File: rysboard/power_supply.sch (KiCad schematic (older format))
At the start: 31 parts, among them J19 Fan_Connector, Q3 NST847BDP6T5G, Q4 DMP3036SSD-13, Q5 DMP3036SSD-13, U3 ST1S10, U6 L78L33_SO8

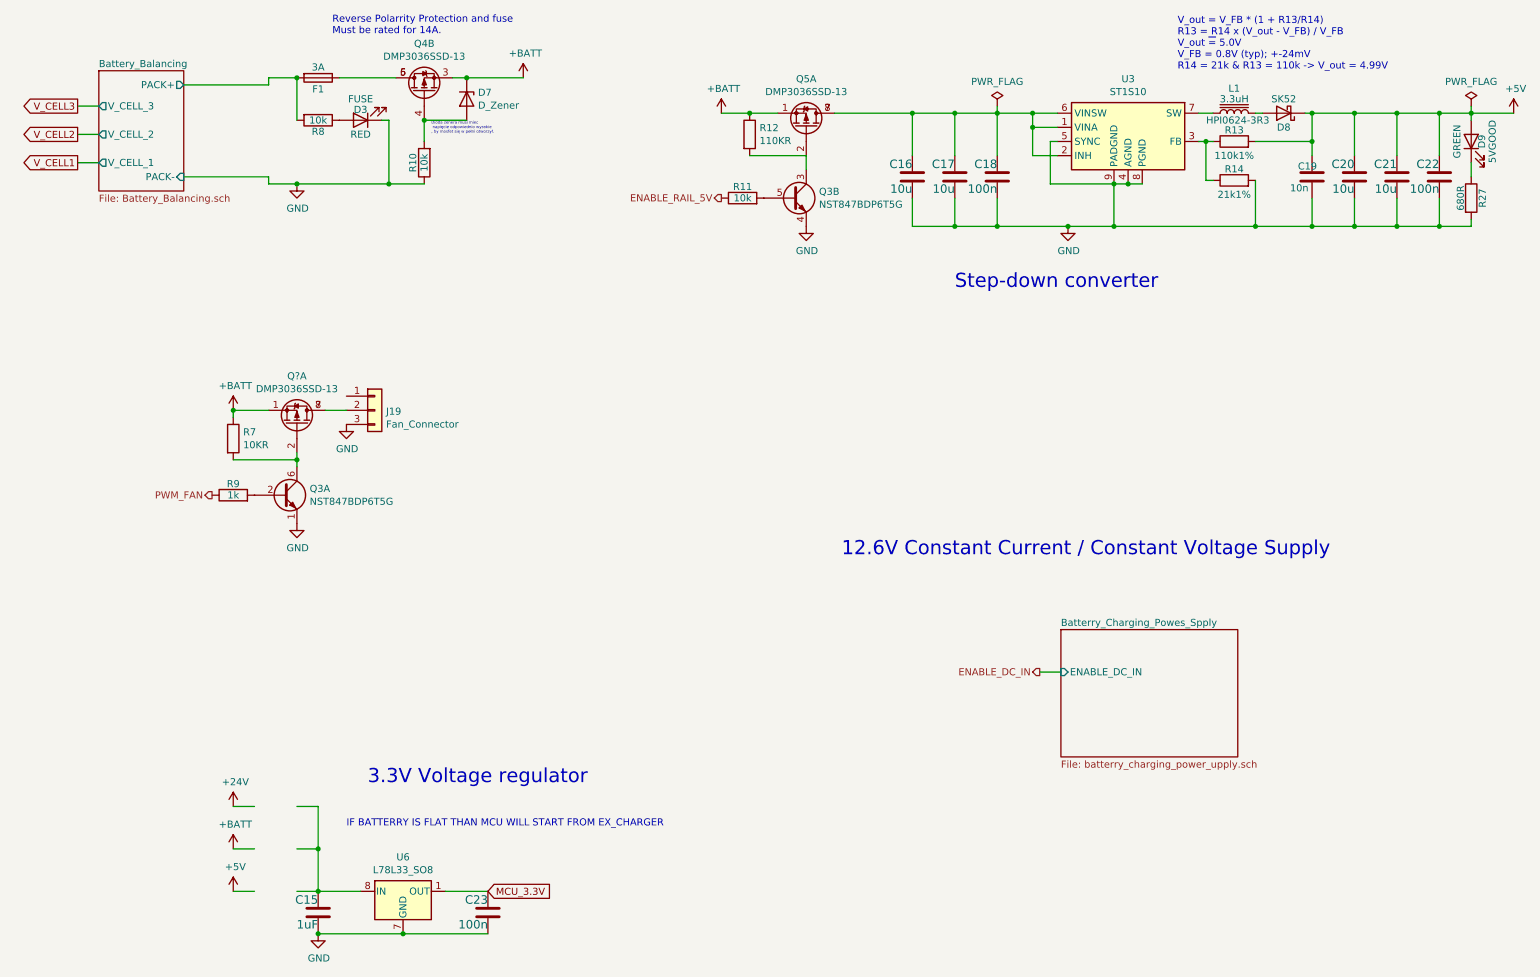
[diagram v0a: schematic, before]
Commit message: more work done
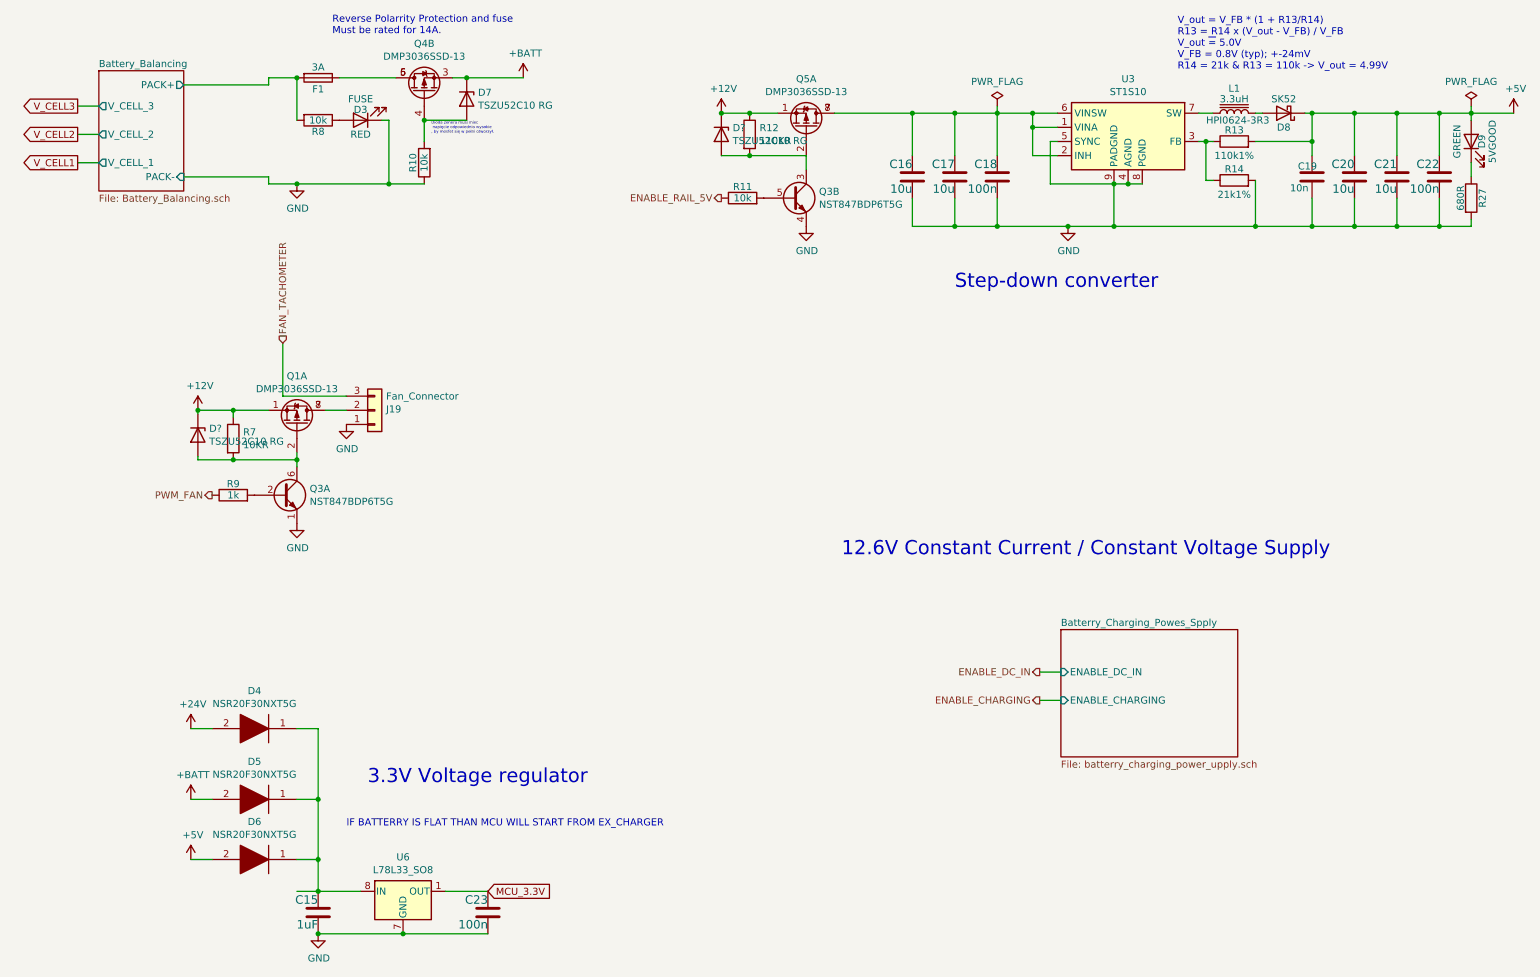
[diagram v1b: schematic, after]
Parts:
- added D4, D5, D6: NSR20F30NXT5G, DSN2_1, symbol SamacSys_Parts:NSR20F30NXT5G
- added D? (x2): TSZU52C10 RG, Diode_SMD:D_0603_1608Metric, symbol Device:D_Zener
- D7: value D_Zener -> TSZU52C10 RG; footprint (none) -> Diode_SMD:D_0603_1608Metric
- gave numbers to parts that had none: 1
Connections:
- net labels added: +12V, ENABLE_CHARGING, FAN_TACHOMETER
- wire segments 101 -> 111
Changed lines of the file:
@@
 P 3600 1250
 F 0 "D7" V 3554 1330 50  0000 L CNN
-F 1 "D_Zener" V 3645 1330 50  0000 L CNN
-F 2 "" H 3600 1250 50  0001 C CNN
+F 1 "TSZU52C10 RG" V 3645 1330 50  0000 L CNN
+F 2 "Diode_SMD:D_0603_1608Metric" H 3600 1250 50  0001 C CNN
 F 3 "~" H 3600 1250 50  0001 C CNN
 	1    3600 1250
@@
 Text Notes 2650 800  0    50   ~ 0
 Reverse Polarrity Protection and fuse\nMust be rated for 14A.\n
-Wire Wire Line
-	2400 6550 2550 6550
-Wire Wire Line
-	2550 6550 2550 6850
 Text Notes 2750 6400 0    50   ~ 0
 IF BATTERRY IS FLAT THAN MCU WILL START FROM EX_CHARGER\n
@@
 F1 "batterry_charging_power_upply.sch" 50
 F2 "ENABLE_DC_IN" I L 7800 5300 50
+F3 "ENABLE_CHARGING" I L 7800 5500 50
 $EndSheet
 $Comp
@@
 	6200 1350 6750 1350
 Connection ~ 6750 1350
-$Comp
-L power:+BATT #PWR035
-U 1 1 605D53D0
-P 5400 1350
-F 0 "#PWR035" H 5400 1200 50  0001 C CNN
-F 1 "+BATT" H 5415 1523 50  0000 C CNN
-F 2 "" H 5400 1350 50  0001 C CNN
-F 3 "" H 5400 1350 50  0001 C CNN
-	1    5400 1350
-	1    0    0    -1
-$EndComp
 $Comp
 L Device:R R12
@@
 Wire Wire Line
 	1950 3450 1950 3500
-$Comp
-L power:+BATT #PWR024
-U 1 1 60610E26
-P 1950 3450
-F 0 "#PWR024" H 1950 3300 50  0001 C CNN
-F 1 "+BATT" H 1965 3623 50  0000 C CNN
-F 2 "" H 1950 3450 50  0001 C CNN
-F 3 "" H 1950 3450 50  0001 C CNN
-	1    1950 3450
-	1    0    0    -1
-$EndComp
 Connection ~ 1950 3450
 $Comp
@@
 F 3 "~" H 2950 3450 50  0001 C CNN
 	1    2950 3450
-	1    0    0    -1
+	1    0    0    1
 $EndComp
 Wire Wire Line
@@
 L power:+BATT #PWR027
 U 1 1 6066923D
-P 1950 6550
-F 0 "#PWR027" H 1950 6400 50  0001 C CNN
-F 1 "+BATT" H 1965 6723 50  0000 C CNN
-F 2 "" H 1950 6550 50  0001 C CNN
-F 3 "" H 1950 6550 50  0001 C CNN
-	1    1950 6550
-	1    0    0    -1
-$EndComp
-Wire Wire Line
-	1950 6550 2100 6550
+P 1650 6200
+F 0 "#PWR027" H 1650 6050 50  0001 C CNN
+F 1 "+BATT" H 1665 6373 50  0000 C CNN
+F 2 "" H 1650 6200 50  0001 C CNN
+F 3 "" H 1650 6200 50  0001 C CNN
+	1    1650 6200
+	1    0    0    -1
+$EndComp
+Wire Wire Line
+	1650 6200 1800 6200
 $Comp
 L power:+24V #PWR025
 U 1 1 606699BF
-P 1950 6250
-F 0 "#PWR025" H 1950 6100 50  0001 C CNN
-F 1 "+24V" H 1965 6423 50  0000 C CNN
-F 2 "" H 1950 6250 50  0001 C CNN
-F 3 "" H 1950 6250 50  0001 C CNN
-	1    1950 6250
-	1    0    0    -1
-$EndComp
-Wire Wire Line
-	1950 6250 2100 6250
-Wire Wire Line
-	2550 6550 2550 6250
-Wire Wire Line
-	2550 6250 2400 6250
-Connection ~ 2550 6550
+P 1650 5700
+F 0 "#PWR025" H 1650 5550 50  0001 C CNN
+F 1 "+24V" H 1665 5873 50  0000 C CNN
+F 2 "" H 1650 5700 50  0001 C CNN
+F 3 "" H 1650 5700 50  0001 C CNN
+	1    1650 5700
+	1    0    0    -1
+$EndComp
+Wire Wire Line
+	1650 5700 1800 5700
+Wire Wire Line
+	2550 5700 2400 5700
 $Comp
 L power:+5V #PWR029
 U 1 1 6067B267
-P 1950 6850
-F 0 "#PWR029" H 1950 6700 50  0001 C CNN
-F 1 "+5V" H 1965 7023 50  0000 C CNN
-F 2 "" H 1950 6850 50  0001 C CNN
-F 3 "" H 1950 6850 50  0001 C CNN
-	1    1950 6850
-	1    0    0    -1
-$EndComp
-Wire Wire Line
-	1950 6850 2100 6850
+P 1650 6625
+F 0 "#PWR029" H 1650 6475 50  0001 C CNN
+F 1 "+5V" H 1665 6798 50  0000 C CNN
+F 2 "" H 1650 6625 50  0001 C CNN
+F 3 "" H 1650 6625 50  0001 C CNN
+	1    1650 6625
+	1    0    0    -1
+$EndComp
+Wire Wire Line
+	1650 6625 1800 6625
 Text HLabel 5400 1950 0    50   Output ~ 0
 ENABLE_RAIL_5V
@@
 $EndComp
 $Comp
-L rysboard:DMP3036SSD-13 Q?
+L rysboard:DMP3036SSD-13 Q1
 U 1 1 605FF267
 P 2400 3550
-F 0 "Q?" V 2742 3550 50  0000 C CNN
+F 0 "Q1" V 2742 3550 50  0000 C CNN
 F 1 "DMP3036SSD-13" V 2651 3550 50  0000 C CNN
 F 2 "Package_SO:SO-8_3.9x4.9mm_P1.27mm" H 2600 3475 50  0001 L CIN
@@
 	0    1    -1   0
 $EndComp
+$Comp
+L SamacSys_Parts:NSR20F30NXT5G D4
+U 1 1 60433DC9
+P 2400 5700
+F 0 "D4" H 2700 5433 50  0000 C CNN
+F 1 "NSR20F30NXT5G" H 2700 5524 50  0000 C CNN
+F 2 "DSN2_1" H 2850 5700 50  0001 L CNN
+F 3 "http://www.onsemi.com/pub/Collateral/NSR20F30-D.PDF" H 2850 5600 50  0001 L CNN
+F 4 "ON SEMICONDUCTOR - NSR20F30NXT5G - DIODE, SCHOTTKY, 2A, 30V, 0603" H 2850 5500 50  0001 L CNN "Description"
+F 5 "" H 2850 5400 50  0001 L CNN "Height"
+F 6 "863-NSR20F30NXT5G" H 2850 5300 50  0001 L CNN "Mouser Part Number"
+F 7 "https://www.mouser.co.uk/ProductDetail/ON-Semiconductor/NSR20F30NXT5G/?qs=3ezCrKCRT5K%2FARb%252BJ8n8Hg%3D%3D" H 2850 5200 50  0001 L CNN "Mouser Price/Stock"
+F 8 "ON Semiconductor" H 2850 5100 50  0001 L CNN "Manufacturer_Name"
+F 9 "NSR20F30NXT5G" H 2850 5000 50  0001 L CNN "Manufacturer_Part_Number"
+	1    2400 5700
+	-1   0    0    1
+$EndComp
+Wire Wire Line
+	2550 5700 2550 6200
+$Comp
+L SamacSys_Parts:NSR20F30NXT5G D5
+U 1 1 6044F2F9
+P 2400 6200
+F 0 "D5" H 2700 5933 50  0000 C CNN
+F 1 "NSR20F30NXT5G" H 2700 6024 50  0000 C CNN
+F 2 "DSN2_1" H 2850 6200 50  0001 L CNN
+F 3 "http://www.onsemi.com/pub/Collateral/NSR20F30-D.PDF" H 2850 6100 50  0001 L CNN
+F 4 "ON SEMICONDUCTOR - NSR20F30NXT5G - DIODE, SCHOTTKY, 2A, 30V, 0603" H 2850 6000 50  0001 L CNN "Description"
+F 5 "" H 2850 5900 50  0001 L CNN "Height"
+F 6 "863-NSR20F30NXT5G" H 2850 5800 50  0001 L CNN "Mouser Part Number"
+F 7 "https://www.mouser.co.uk/ProductDetail/ON-Semiconductor/NSR20F30NXT5G/?qs=3ezCrKCRT5K%2FARb%252BJ8n8Hg%3D%3D" H 2850 5700 50  0001 L CNN "Mouser Price/Stock"
+F 8 "ON Semiconductor" H 2850 5600 50  0001 L CNN "Manufacturer_Name"
+F 9 "NSR20F30NXT5G" H 2850 5500 50  0001 L CNN "Manufacturer_Part_Number"
+	1    2400 6200
+	-1   0    0    1
+$EndComp
+$Comp
+L SamacSys_Parts:NSR20F30NXT5G D6
+U 1 1 6044F644
+P 2400 6625
+F 0 "D6" H 2700 6358 50  0000 C CNN
+F 1 "NSR20F30NXT5G" H 2700 6449 50  0000 C CNN
+F 2 "DSN2_1" H 2850 6625 50  0001 L CNN
+F 3 "http://www.onsemi.com/pub/Collateral/NSR20F30-D.PDF" H 2850 6525 50  0001 L CNN
+F 4 "ON SEMICONDUCTOR - NSR20F30NXT5G - DIODE, SCHOTTKY, 2A, 30V, 0603" H 2850 6425 50  0001 L CNN "Description"
+F 5 "" H 2850 6325 50  0001 L CNN "Height"
+F 6 "863-NSR20F30NXT5G" H 2850 6225 50  0001 L CNN "Mouser Part Number"
+F 7 "https://www.mouser.co.uk/ProductDetail/ON-Semiconductor/NSR20F30NXT5G/?qs=3ezCrKCRT5K%2FARb%252BJ8n8Hg%3D%3D" H 2850 6125 50  0001 L CNN "Mouser Price/Stock"
+F 8 "ON Semiconductor" H 2850 6025 50  0001 L CNN "Manufacturer_Name"
+F 9 "NSR20F30NXT5G" H 2850 5925 50  0001 L CNN "Manufacturer_Part_Number"
+	1    2400 6625
+	-1   0    0    1
+$EndComp
+Wire Wire Line
+	2400 6200 2550 6200
+Connection ~ 2550 6200
+Wire Wire Line
+	2550 6200 2550 6625
+Wire Wire Line
+	2400 6625 2550 6625
+Connection ~ 2550 6625
+Wire Wire Line
+	2550 6625 2550 6850
+Text HLabel 7650 5500 0    50   Output ~ 0
+ENABLE_CHARGING
+Wire Wire Line
+	7650 5500 7800 5500
+$Comp
+L Device:D_Zener D?
+U 1 1 604A195B
+P 5400 1500
+F 0 "D?" V 5354 1580 50  0000 L CNN
+F 1 "TSZU52C10 RG" V 5445 1580 50  0000 L CNN
+F 2 "Diode_SMD:D_0603_1608Metric" H 5400 1500 50  0001 C CNN
+F 3 "~" H 5400 1500 50  0001 C CNN
+	1    5400 1500
+	0    1    1    0
+$EndComp
+Wire Wire Line
+	5400 1650 5600 1650
+Connection ~ 5600 1650
+$Comp
+L Device:D_Zener D?
+U 1 1 604A5F28
+P 1700 3625
+F 0 "D?" V 1654 3705 50  0000 L CNN
+F 1 "TSZU52C10 RG" V 1745 3705 50  0000 L CNN
+F 2 "Diode_SMD:D_0603_1608Metric" H 1700 3625 50  0001 C CNN
+F 3 "~" H 1700 3625 50  0001 C CNN
+	1    1700 3625
+	0    1    1    0
+$EndComp
+Wire Wire Line
+	1700 3775 1700 3800
+Wire Wire Line
+	1700 3800 1950 3800
+Connection ~ 1950 3800
+Wire Wire Line
+	1700 3475 1700 3450
+Wire Wire Line
+	1700 3450 1950 3450
+Text HLabel 2300 2975 1    50   Input ~ 0
+FAN_TACHOMETER
+Wire Wire Line
+	2300 2975 2300 3350
+Wire Wire Line
+	2300 3350 2750 3350
+$Comp
+L power:+12V #PWR?
+U 1 1 604BD223
+P 1700 3450
+F 0 "#PWR?" H 1700 3300 50  0001 C CNN
+F 1 "+12V" H 1715 3623 50  0000 C CNN
+F 2 "" H 1700 3450 50  0001 C CNN
+F 3 "" H 1700 3450 50  0001 C CNN
+	1    1700 3450
+	1    0    0    -1
+$EndComp
+Connection ~ 1700 3450
+$Comp
+L power:+12V #PWR?
+U 1 1 604BD987
+P 5400 1350
+F 0 "#PWR?" H 5400 1200 50  0001 C CNN
+F 1 "+12V" H 5415 1523 50  0000 C CNN
+F 2 "" H 5400 1350 50  0001 C CNN
+F 3 "" H 5400 1350 50  0001 C CNN
+	1    5400 1350
+	1    0    0    -1
+$EndComp
+Connection ~ 5400 1350
 $EndSCHEMATC

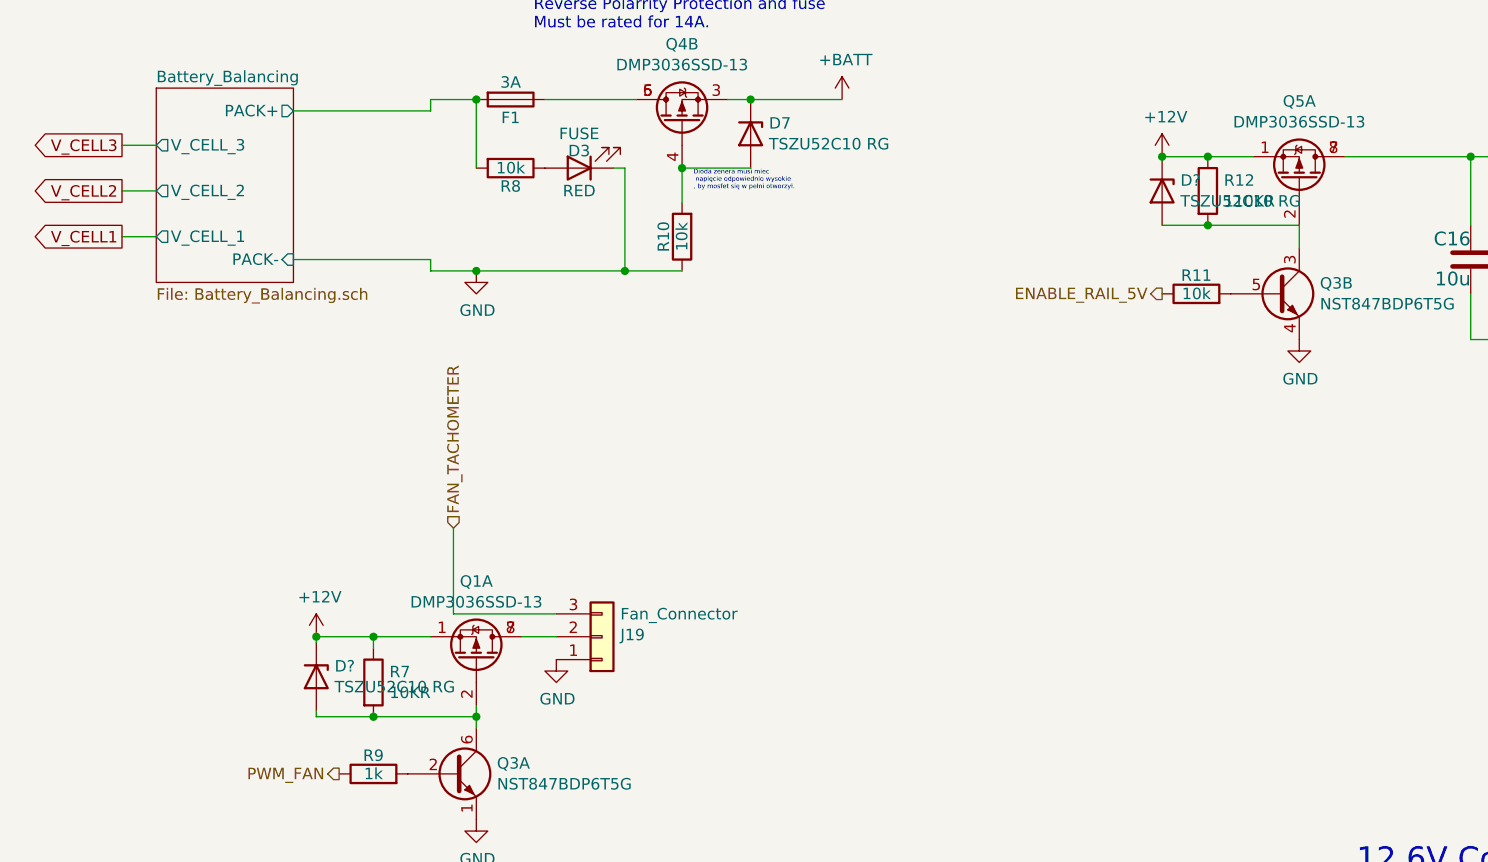
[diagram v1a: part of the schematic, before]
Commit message: more footprints
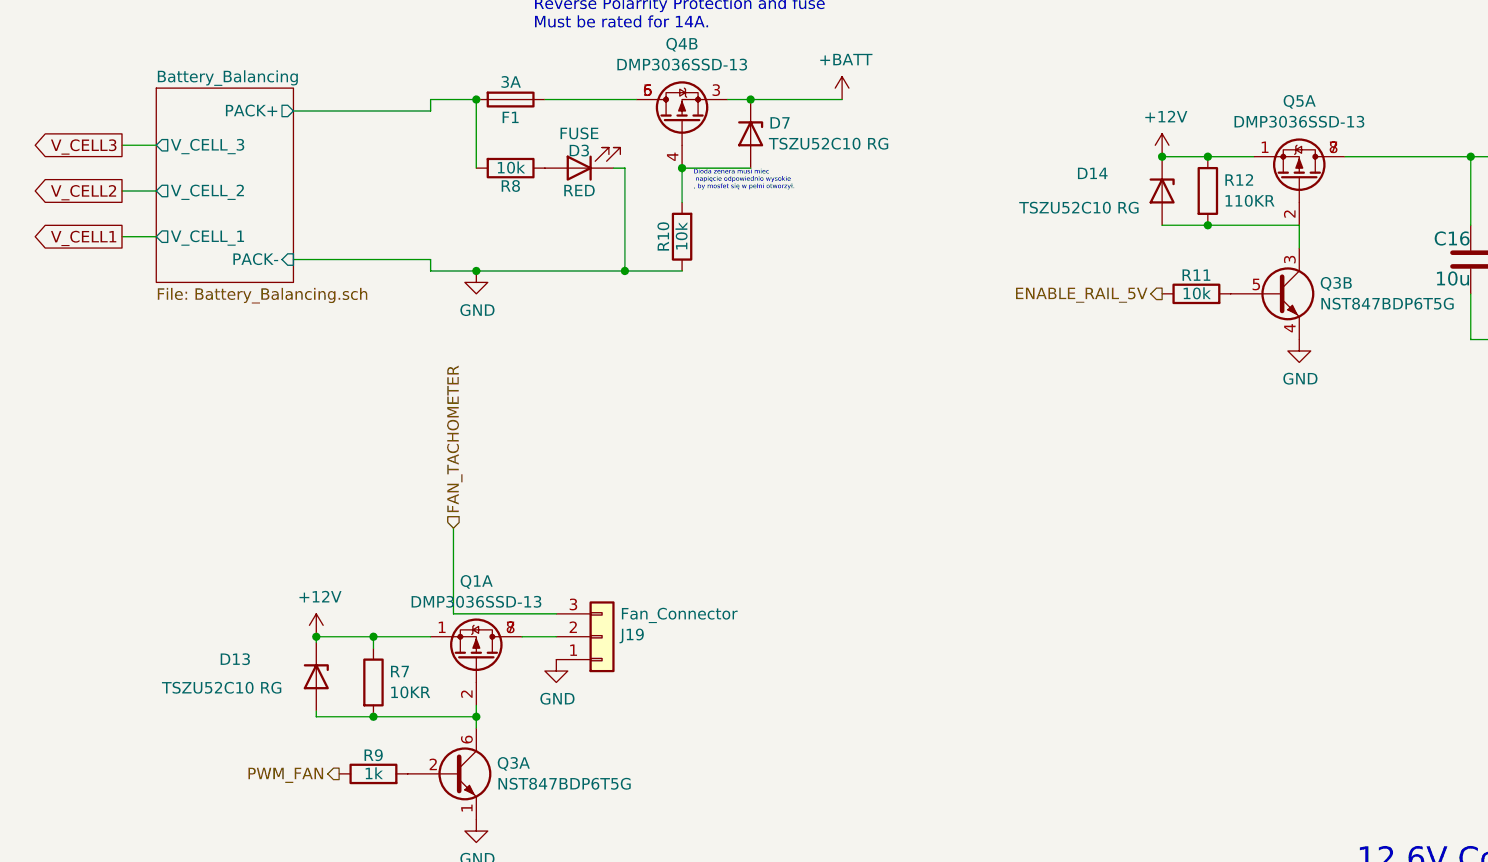
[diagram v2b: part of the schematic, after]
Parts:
- D4, D5, D6: footprint DSN2_1 -> SamacSys_Parts:DSN2_1
- gave numbers to parts that had none: 2
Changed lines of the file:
@@
 F 0 "D4" H 2700 5433 50  0000 C CNN
 F 1 "NSR20F30NXT5G" H 2700 5524 50  0000 C CNN
-F 2 "DSN2_1" H 2850 5700 50  0001 L CNN
+F 2 "SamacSys_Parts:DSN2_1" H 2850 5700 50  0001 L CNN
 F 3 "http://www.onsemi.com/pub/Collateral/NSR20F30-D.PDF" H 2850 5600 50  0001 L CNN
 F 4 "ON SEMICONDUCTOR - NSR20F30NXT5G - DIODE, SCHOTTKY, 2A, 30V, 0603" H 2850 5500 50  0001 L CNN "Description"
@@
 F 0 "D5" H 2700 5933 50  0000 C CNN
 F 1 "NSR20F30NXT5G" H 2700 6024 50  0000 C CNN
-F 2 "DSN2_1" H 2850 6200 50  0001 L CNN
+F 2 "SamacSys_Parts:DSN2_1" H 2850 6200 50  0001 L CNN
 F 3 "http://www.onsemi.com/pub/Collateral/NSR20F30-D.PDF" H 2850 6100 50  0001 L CNN
 F 4 "ON SEMICONDUCTOR - NSR20F30NXT5G - DIODE, SCHOTTKY, 2A, 30V, 0603" H 2850 6000 50  0001 L CNN "Description"
@@
 F 0 "D6" H 2700 6358 50  0000 C CNN
 F 1 "NSR20F30NXT5G" H 2700 6449 50  0000 C CNN
-F 2 "DSN2_1" H 2850 6625 50  0001 L CNN
+F 2 "SamacSys_Parts:DSN2_1" H 2850 6625 50  0001 L CNN
 F 3 "http://www.onsemi.com/pub/Collateral/NSR20F30-D.PDF" H 2850 6525 50  0001 L CNN
 F 4 "ON SEMICONDUCTOR - NSR20F30NXT5G - DIODE, SCHOTTKY, 2A, 30V, 0603" H 2850 6425 50  0001 L CNN "Description"
@@
 	7650 5500 7800 5500
 $Comp
-L Device:D_Zener D?
+L Device:D_Zener D14
 U 1 1 604A195B
 P 5400 1500
-F 0 "D?" V 5354 1580 50  0000 L CNN
-F 1 "TSZU52C10 RG" V 5445 1580 50  0000 L CNN
+F 0 "D14" V 5325 1125 50  0000 L CNN
+F 1 "TSZU52C10 RG" V 5475 875 50  0000 L CNN
 F 2 "Diode_SMD:D_0603_1608Metric" H 5400 1500 50  0001 C CNN
 F 3 "~" H 5400 1500 50  0001 C CNN
@@
 Connection ~ 5600 1650
 $Comp
-L Device:D_Zener D?
+L Device:D_Zener D13
 U 1 1 604A5F28
 P 1700 3625
-F 0 "D?" V 1654 3705 50  0000 L CNN
-F 1 "TSZU52C10 RG" V 1745 3705 50  0000 L CNN
+F 0 "D13" V 1625 3200 50  0000 L CNN
+F 1 "TSZU52C10 RG" V 1750 2950 50  0000 L CNN
 F 2 "Diode_SMD:D_0603_1608Metric" H 1700 3625 50  0001 C CNN
 F 3 "~" H 1700 3625 50  0001 C CNN
@@
 	2300 3350 2750 3350
 $Comp
-L power:+12V #PWR?
+L power:+12V #PWR0104
 U 1 1 604BD223
 P 1700 3450
-F 0 "#PWR?" H 1700 3300 50  0001 C CNN
+F 0 "#PWR0104" H 1700 3300 50  0001 C CNN
 F 1 "+12V" H 1715 3623 50  0000 C CNN
 F 2 "" H 1700 3450 50  0001 C CNN
@@
 Connection ~ 1700 3450
 $Comp
-L power:+12V #PWR?
+L power:+12V #PWR0105
 U 1 1 604BD987
 P 5400 1350
-F 0 "#PWR?" H 5400 1200 50  0001 C CNN
+F 0 "#PWR0105" H 5400 1200 50  0001 C CNN
 F 1 "+12V" H 5415 1523 50  0000 C CNN
 F 2 "" H 5400 1350 50  0001 C CNN
